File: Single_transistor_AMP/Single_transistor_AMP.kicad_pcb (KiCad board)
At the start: 2 copper layers, 50 x 43.3 mm, 12 parts, among them J1 Barosana un ieeja, J2 Izeja, J3 Stiprinajums1, J4 Stiprinajums2, J5 Stiprinajums3, Q1 BC547

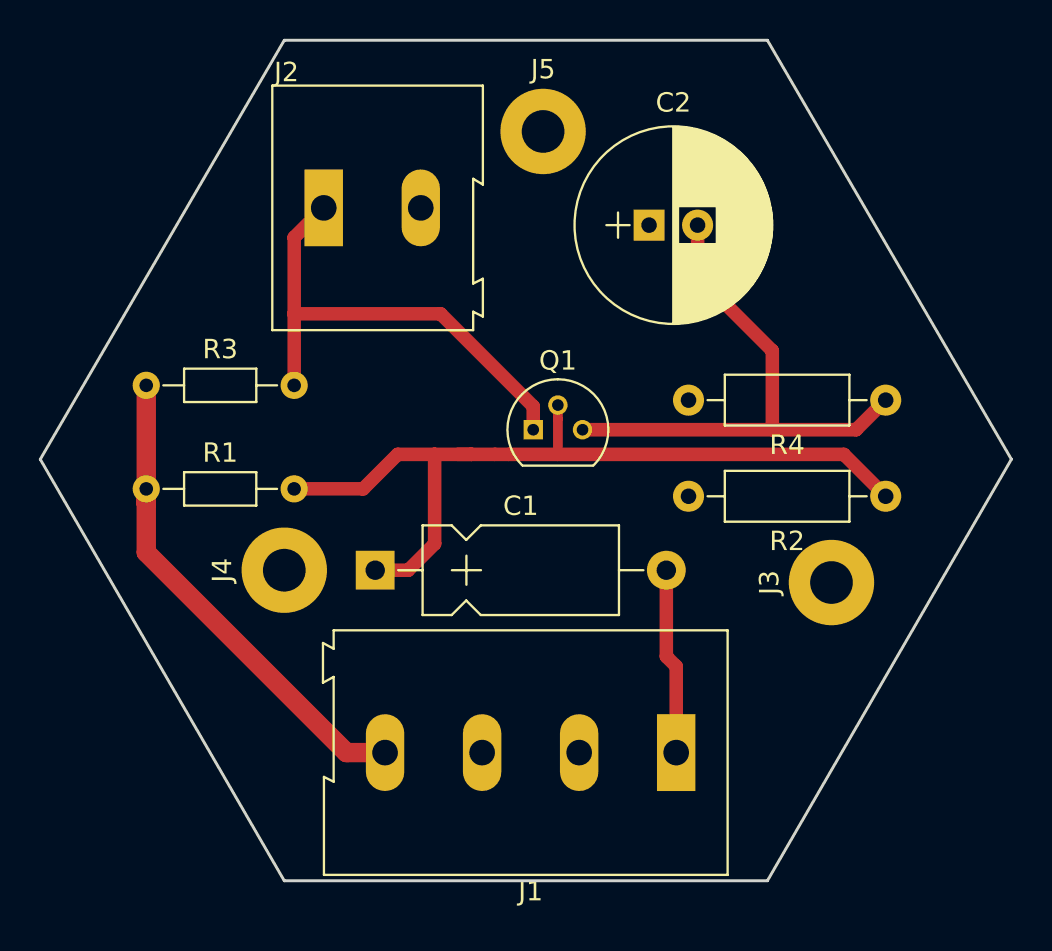
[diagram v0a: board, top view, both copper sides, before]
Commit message: Single_transistor_AMP 2. iteraacija
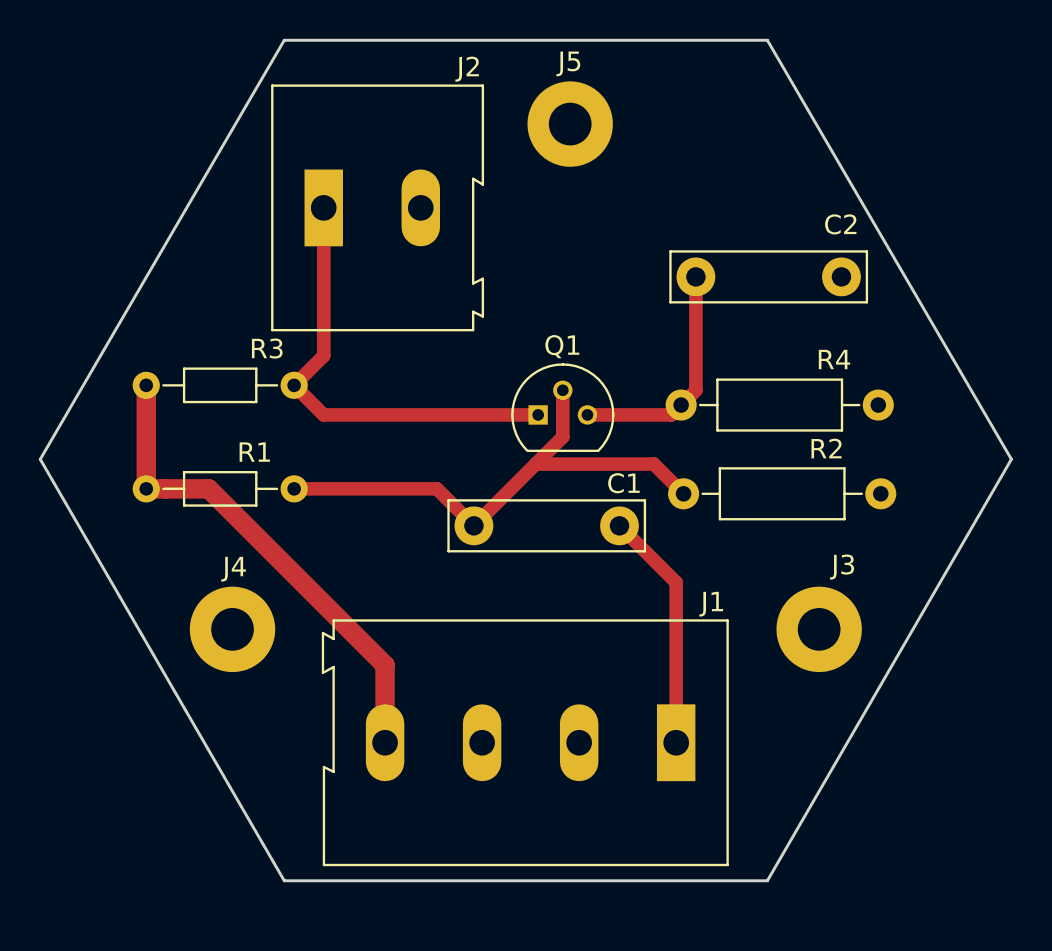
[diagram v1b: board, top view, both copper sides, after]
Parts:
- C1: footprint Capacitors_THT:CP_Axial_L10.0mm_D4.5mm_P15.00mm_Horizontal -> Capacitors_THT:C_Rect_L10.0mm_W2.5mm_P7.50mm_MKS4
- C2: footprint Capacitors_THT:CP_Radial_D10.0mm_P2.50mm -> Capacitors_THT:C_Rect_L10.0mm_W2.5mm_P7.50mm_MKS4
- moved R4 10.5 mm to (113.9, 136.9), turned to 0 degrees
- moved R2 10.4 mm to (114.0, 141.5), turned to 0 degrees
- moved C2 10.3 mm to (122.2, 130.3), turned to 180 degrees
- moved C1 5.58 mm to (103.2, 143.1)
- moved J4 4.05 mm to (90.8, 148.5), turned to 0 degrees
- moved J3 2.50 mm to (121.0, 148.5), turned to 0 degrees
- moved J5 1.45 mm to (108.2, 122.4)
- moved Q1 0.80 mm to (106.6, 137.4)
- moved J1 0.51 mm to (113.7, 154.3)
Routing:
- net Net-(C2-Pad2): track 28.4 -> 12.0 mm
- net Net-(C1-Pad1): track 43.6 -> 27.2 mm
- net Net-(J2-Pad1): track 25.3 -> 23.0 mm
- net Net-(C1-Pad2): track 9.61 -> 11.4 mm
- net +9V: track 25.9 -> 24.4 mm
